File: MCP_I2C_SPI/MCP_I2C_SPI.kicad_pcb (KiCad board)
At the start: 2 copper layers, 122 x 95 mm, 50 parts, among them J1 GPA, J10 VCC, J11 GND, J12 I2C, J13 Interrupt0, J14 A2, J15 A1, J16 A0, J17 SDA, J18 SCK, J19 INTA, J2 GPB, J20 INTB, J21 V0, J22 Ext, J23 SPI, J24 InterruptS, J25 A2, J27 GPB, J28 GPA, J29 A1, J3 Data, J31 A0, J32 INTA, J33 INTB, J4 Control, J5 Zlacze_LCD, J6 VSS, J7 K, J8 VDD, J9 A, U1 MCP23017_SP, U2 MCP23017_SP

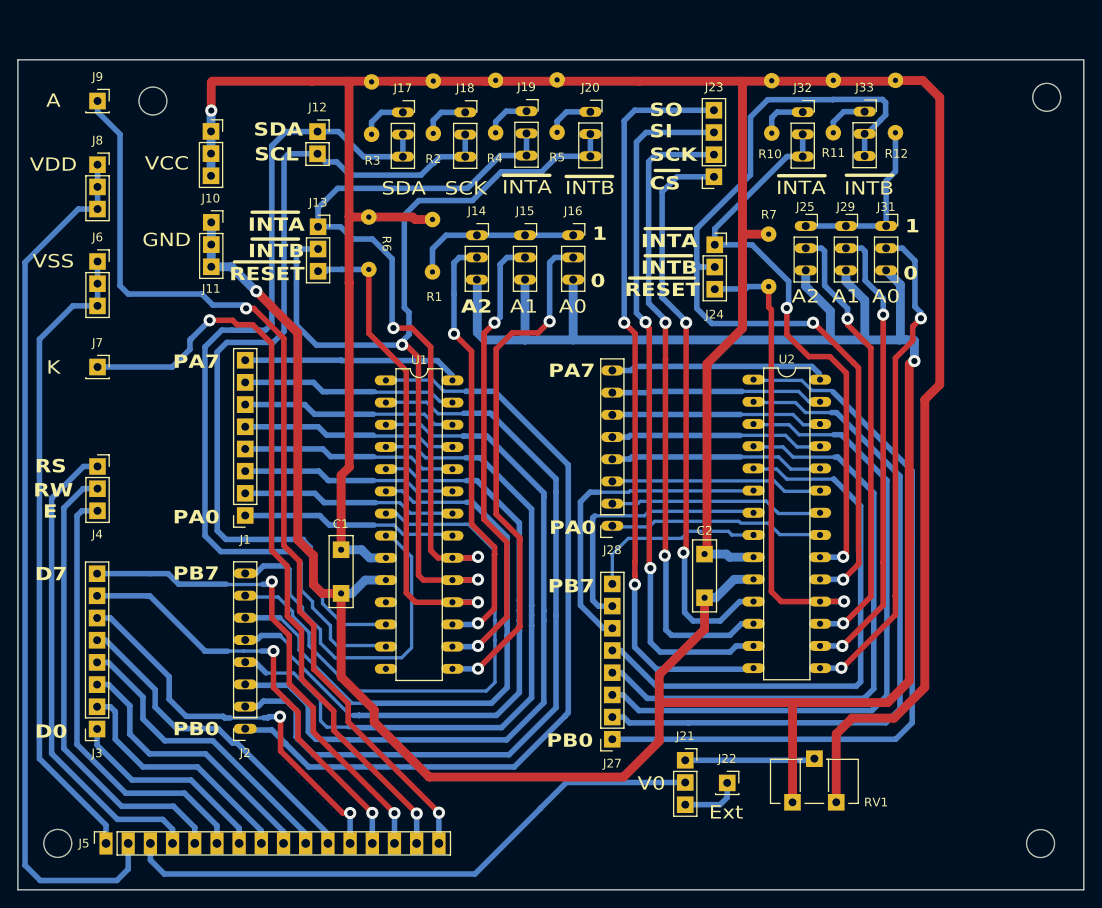
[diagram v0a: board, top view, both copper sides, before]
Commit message: MCP_I2C_SPI_PCB_V6
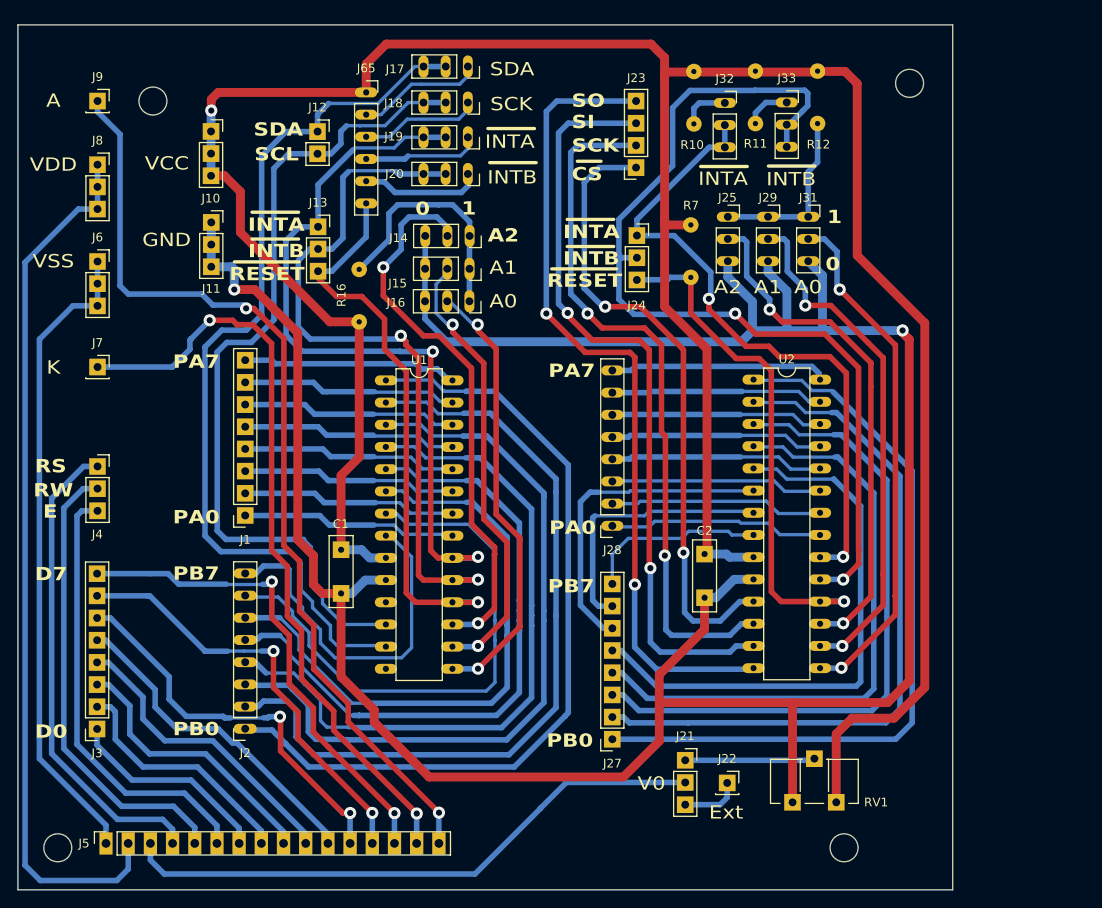
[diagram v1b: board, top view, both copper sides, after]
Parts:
- removed R1, R4, R5, R6: 10k, Library:Resistor_6mm
- removed R2, R3: 4k7, Library:Resistor_6mm
- added J65: SIL6, Connector_PinSocket_2.54mm:PinSocket_1x06_P2.54mm_Vertical, F.Cu at (91.8, 29.0)
- added R16: 10k, Library:Resistor_6mm, F.Cu at (91.0, 55.3)
- moved REF** 22.5 mm to (146.5, 115.5)
- moved REF** 15.8 mm to (154.0, 28.0)
- moved J20 15.7 mm to (103.4, 38.4), turned to -90 degrees
- moved J16 14.1 mm to (103.6, 52.9), turned to -90 degrees
- moved J17 9.10 mm to (103.4, 26.1), turned to -90 degrees
- moved J32 8.98 mm to (132.9, 30.2)
- moved R10 8.98 mm to (129.3, 26.6)
- moved R12 8.98 mm to (143.5, 26.6)
- moved J23 8.98 mm to (122.7, 37.6)
- moved J24 8.98 mm to (122.8, 45.4)
- moved J25 8.98 mm to (133.2, 43.3)
- moved J29 8.98 mm to (137.8, 43.3)
- moved J31 8.98 mm to (142.4, 43.3)
- moved J33 8.98 mm to (139.9, 30.2)
- moved R11 8.98 mm to (136.4, 26.6)
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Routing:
- net INTB0: track 103.5 -> 83.7 mm
- net Net-(J14-Pin_2): track 50.0 -> 63.8 mm
- net INTBS: track 99.4 -> 108.8 mm
- net Net-(J17-Pin_1): track 5.43 -> 14.6 mm
- net RESET0: track 56.3 -> 65.3 mm
- net Net-(J16-Pin_2): track 59.7 -> 50.9 mm
- net Net-(J20-Pin_1): track 5.52 -> 13.9 mm
- net INTAS: track 66.7 -> 75.0 mm
- net Net-(J18-Pin_1): track 5.53 -> 13.8 mm
- net SI: track 79.8 -> 88.0 mm
- net Net-(J19-Pin_1): track 5.29 -> 13.4 mm
- net +5V: track 317.5 -> 309.5 mm
- net Net-(J14-Pin_1): track 19.4 -> 27.4 mm
- net Net-(J25-Pin_2): track 51.3 -> 59.3 mm
- net SO: track 86.3 -> 94.0 mm
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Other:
- board size 122 x 95 mm -> 107 x 99 mm

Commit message: Płytka MCP_I2C_SPI_V7
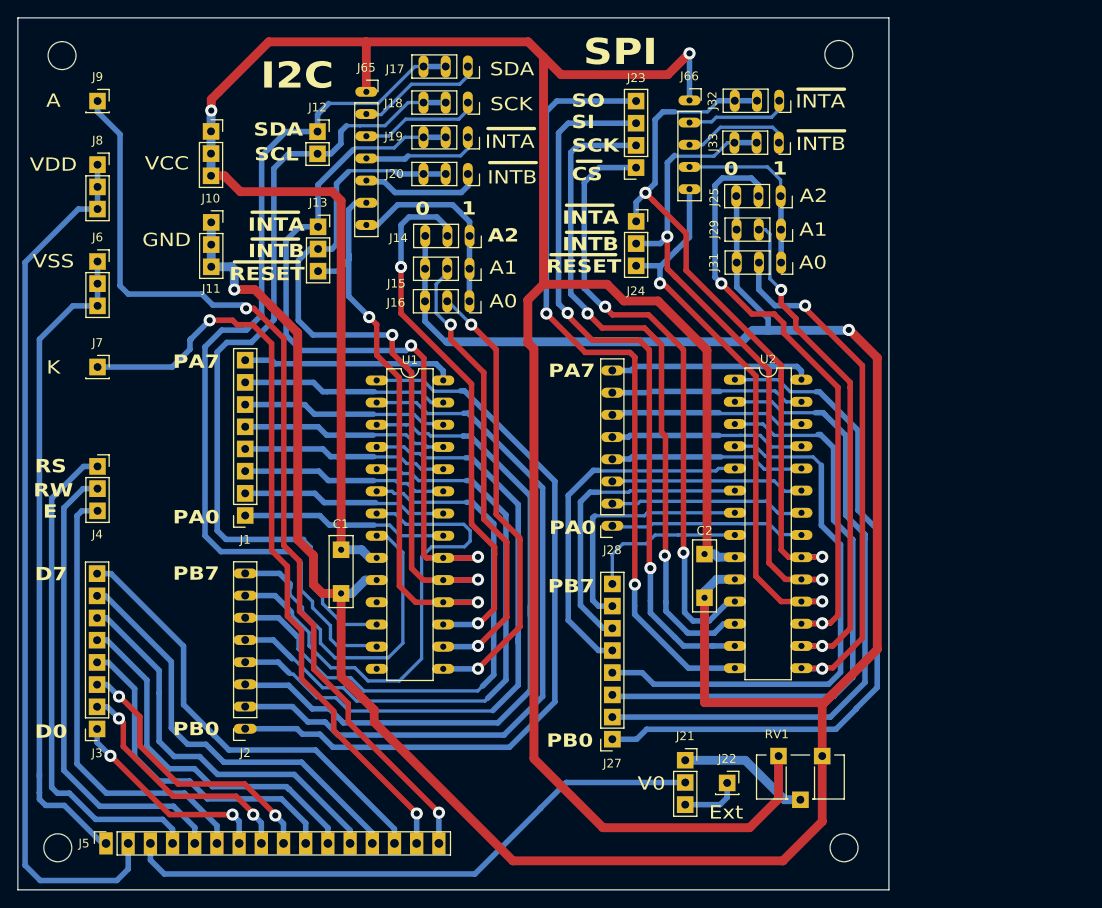
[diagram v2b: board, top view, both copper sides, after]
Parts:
- removed R10, R11, R12, R16, R7: 10k, Library:Resistor_6mm
- added J66: SIL5, Connector_PinSocket_2.54mm:PinSocket_1x05_P2.54mm_Vertical, F.Cu at (128.8, 29.9)
- J65: value SIL6 -> SIL7; footprint Connector_PinSocket_2.54mm:PinSocket_1x06_P2.54mm_Vertical -> Connector_PinSocket_2.54mm:PinSocket_1x07_P2.54mm_Vertical
- moved REF** 11.6 mm to (57.0, 24.8)
- moved REF** 8.75 mm to (145.9, 24.7)
- moved J25 6.49 mm to (139.2, 40.9), turned to -90 degrees
- moved RV1 6.29 mm to (144.0, 105.0), turned to -90 degrees
- moved J32 6.22 mm to (139.1, 30.0), turned to -90 degrees
- moved J31 6.09 mm to (139.3, 48.5), turned to -90 degrees
- moved J33 4.69 mm to (139.0, 34.8), turned to -90 degrees
- moved U2 2.13 mm to (134.0, 61.9)
- moved J29 2.08 mm to (139.3, 44.7), turned to -90 degrees
- moved J24 1.63 mm to (122.7, 43.8)
- moved U1 1.05 mm to (93.0, 62.0)
- moved J65 0.07 mm to (91.8, 29.0)
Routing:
- net INTBS: track 108.8 -> 75.3 mm
- net Net-(J27-Pin_5): track 65.3 -> 41.2 mm
- net Net-(J25-Pin_2): track 59.3 -> 70.8 mm
- net GND: track 310.9 -> 302.5 mm
- net Net-(J2-Pin_2): track 91.8 -> 84.2 mm
- net Net-(J27-Pin_4): track 70.0 -> 62.7 mm
- net Net-(J27-Pin_3): track 75.6 -> 68.2 mm
- net Net-(J33-Pin_1): track 5.30 -> 12.4 mm
- net Net-(J2-Pin_7): track 64.1 -> 57.1 mm
- net Net-(J27-Pin_1): track 86.7 -> 79.9 mm
- net Net-(J27-Pin_2): track 80.9 -> 74.0 mm
- net Net-(J32-Pin_1): track 5.59 -> 12.0 mm
- net Net-(J2-Pin_1): track 94.7 -> 88.9 mm
- net Net-(J2-Pin_3): track 85.8 -> 80.2 mm
- net RESETS: track 59.2 -> 64.8 mm, vias 1 -> 2
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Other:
- board size 107 x 99 mm -> 99.7 x 99.8 mm
- board text added: "I2C"
- board text added: "SPI"
